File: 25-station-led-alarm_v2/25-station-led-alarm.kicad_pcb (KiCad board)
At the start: 2 copper layers, 43 x 73 mm, 31 parts, among them J1 Conn_02x03_Counter_Clockwise, Q1 Q_NMOS_DGS, Q2 Q_NMOS_DGS, Q3 Q_NMOS_DGS

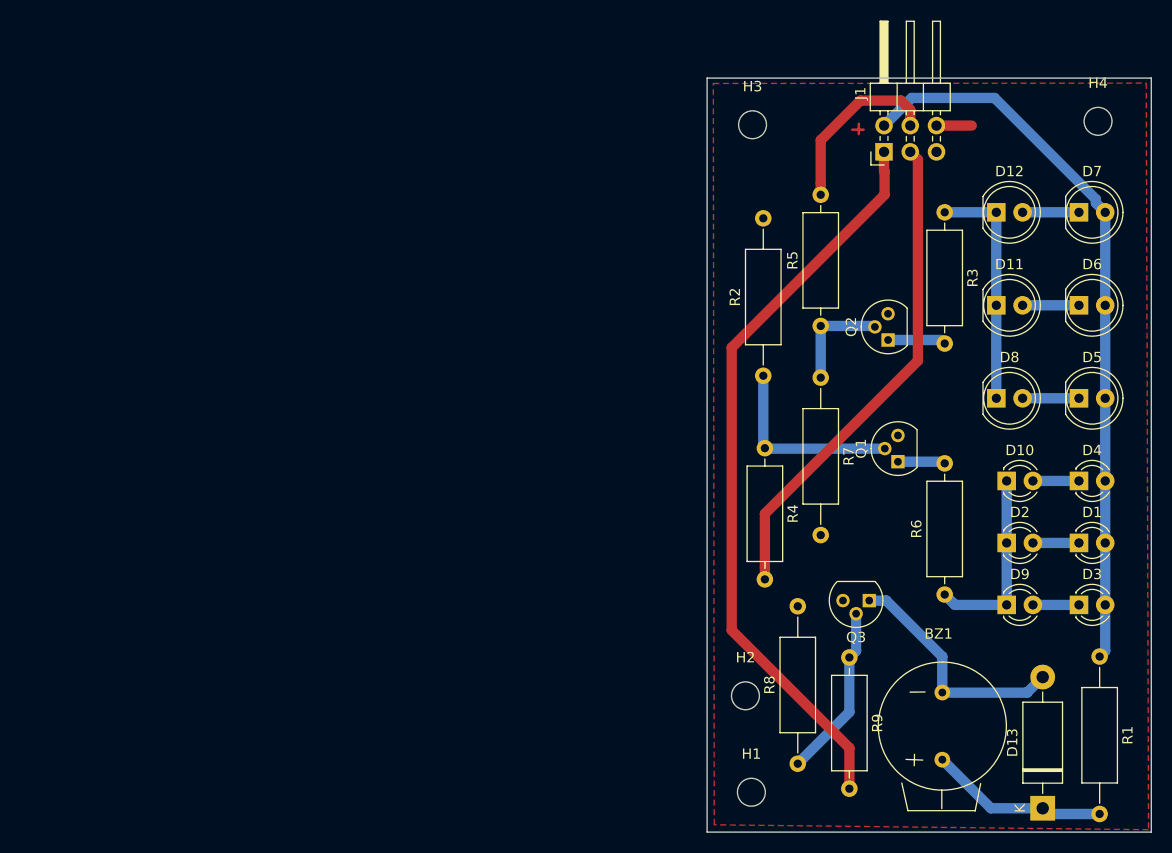
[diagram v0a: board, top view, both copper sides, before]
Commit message: r
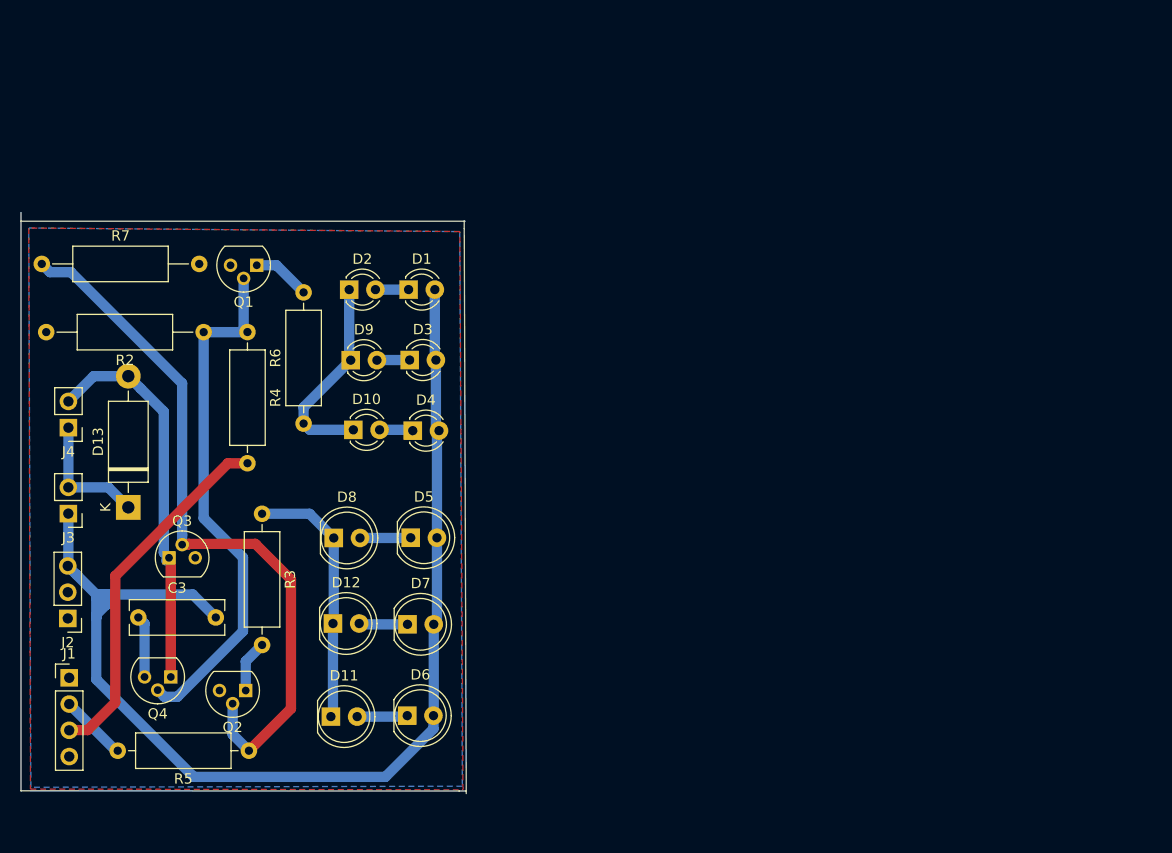
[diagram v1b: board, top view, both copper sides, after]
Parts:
- removed BZ1: Buzzer, Buzzer_Beeper:resita_buzzer
- removed H1, H2, H3, H4: MountingHole_Pad, MountingHole:MountingHole_2.7mm_M2.5
- removed R1: R_sound 30k, Resistor_THT:R_Axial_DIN0309_L9.0mm_D3.2mm_P15.24mm_Horizontal
- removed R8: R_gate 10k, Resistor_THT:R_Axial_DIN0309_L9.0mm_D3.2mm_P15.24mm_Horizontal
- removed R9: R_led 15, Resistor_THT:R_Axial_DIN0309_L9.0mm_D3.2mm_P12.70mm_Horizontal
- added C3: C_Small 47, Capacitor_THT:C_Rect_L9.0mm_W3.2mm_P7.50mm_MKT, F.Cu at (68.9, 139.2)
- added J2: Conn_01x03_Female, Connector_PinHeader_2.54mm:PinHeader_1x03_P2.54mm_Vertical, F.Cu at (62.1, 139.3)
- added J3: Conn_01x02_Female, Connector_PinHeader_2.54mm:PinHeader_1x02_P2.54mm_Vertical, F.Cu at (62.2, 129.2)
- added J4: Conn_01x02_Female, Connector_PinHeader_2.54mm:PinHeader_1x02_P2.54mm_Vertical, F.Cu at (62.2, 120.8)
- added Q4: Q_NMOS_DGS, Package_TO_SOT_THT:TO-92, F.Cu at (72.1, 145.0)
- J1: value Conn_02x03_Counter_Clockwise -> Conn_01x04_Female; footprint Connector_PinHeader_2.54mm:PinHeader_2x03_P2.54mm_Horizontal -> Connector_PinHeader_2.54mm:PinHeader_1x04_P2.54mm_Vertical
- moved J1 93.9 mm to (62.3, 145.1), turned to 0 degrees
- moved D13 93.2 mm to (68.0, 128.6)
- moved D7 76.3 mm to (95.0, 139.9)
- moved R7 76.2 mm to (59.6, 105.0), turned to 0 degrees
- moved D6 76.2 mm to (95.0, 148.7)
- moved D11 75.7 mm to (87.6, 148.8)
- moved D12 75.6 mm to (87.8, 139.8)
- moved R3 72.2 mm to (80.9, 129.2)
- moved Q2 70.8 mm to (79.3, 146.3), turned to 180 degrees
- moved D1 69.4 mm to (95.1, 107.5)
- moved D3 69.0 mm to (95.2, 114.3)
- moved R5 69.0 mm to (79.6, 152.1), turned to 180 degrees
- moved D2 68.2 mm to (89.4, 107.5)
- moved Q3 67.9 mm to (71.9, 133.4), turned to 0 degrees
- moved D9 67.8 mm to (89.5, 114.3)
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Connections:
- J1 pad 1: /P3 -> GND
- J1 pad 2: +5V -> /P2
- J1 pad 4: /P2 -> (no net)
- Q3 pad 2: Net-(Q3-Pad2) -> Net-(Q2-Pad2)
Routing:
- net /P3: track 72.5 -> 0.00 mm
- net Net-(Q2-Pad2): track 10.3 -> 69.5 mm
- net +5V: track 70.5 -> 116.8 mm
- net Net-(Q1-Pad2): track 18.7 -> 51.3 mm
- net Net-(Q3-Pad2): track 16.9 -> 0.00 mm
- net Net-(D13-Pad2): track 23.1 -> 38.3 mm
- net /P1: track 47.8 -> 35.1 mm
- net /P2: track 17.4 -> 6.56 mm
- net Net-(D13-Pad1): track 17.4 -> 12.4 mm
- net Net-(D11-Pad1): track 23.0 -> 25.3 mm
- net Net-(D10-Pad1): track 18.4 -> 20.0 mm
- net Net-(D3-Pad1): track 4.46 -> 3.17 mm
- net Net-(D1-Pad1): track 4.46 -> 3.21 mm
- net Net-(D10-Pad2): track 4.46 -> 3.25 mm
- net Net-(Q1-Pad1): track 4.59 -> 5.62 mm
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- added copper zone on B.Cu, net +5V
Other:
- board size 43 x 73 mm -> 43.1 x 56.2 mm
